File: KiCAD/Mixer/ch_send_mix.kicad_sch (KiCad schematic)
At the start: 16 parts, among them U3 NE5532, U7 NE5532

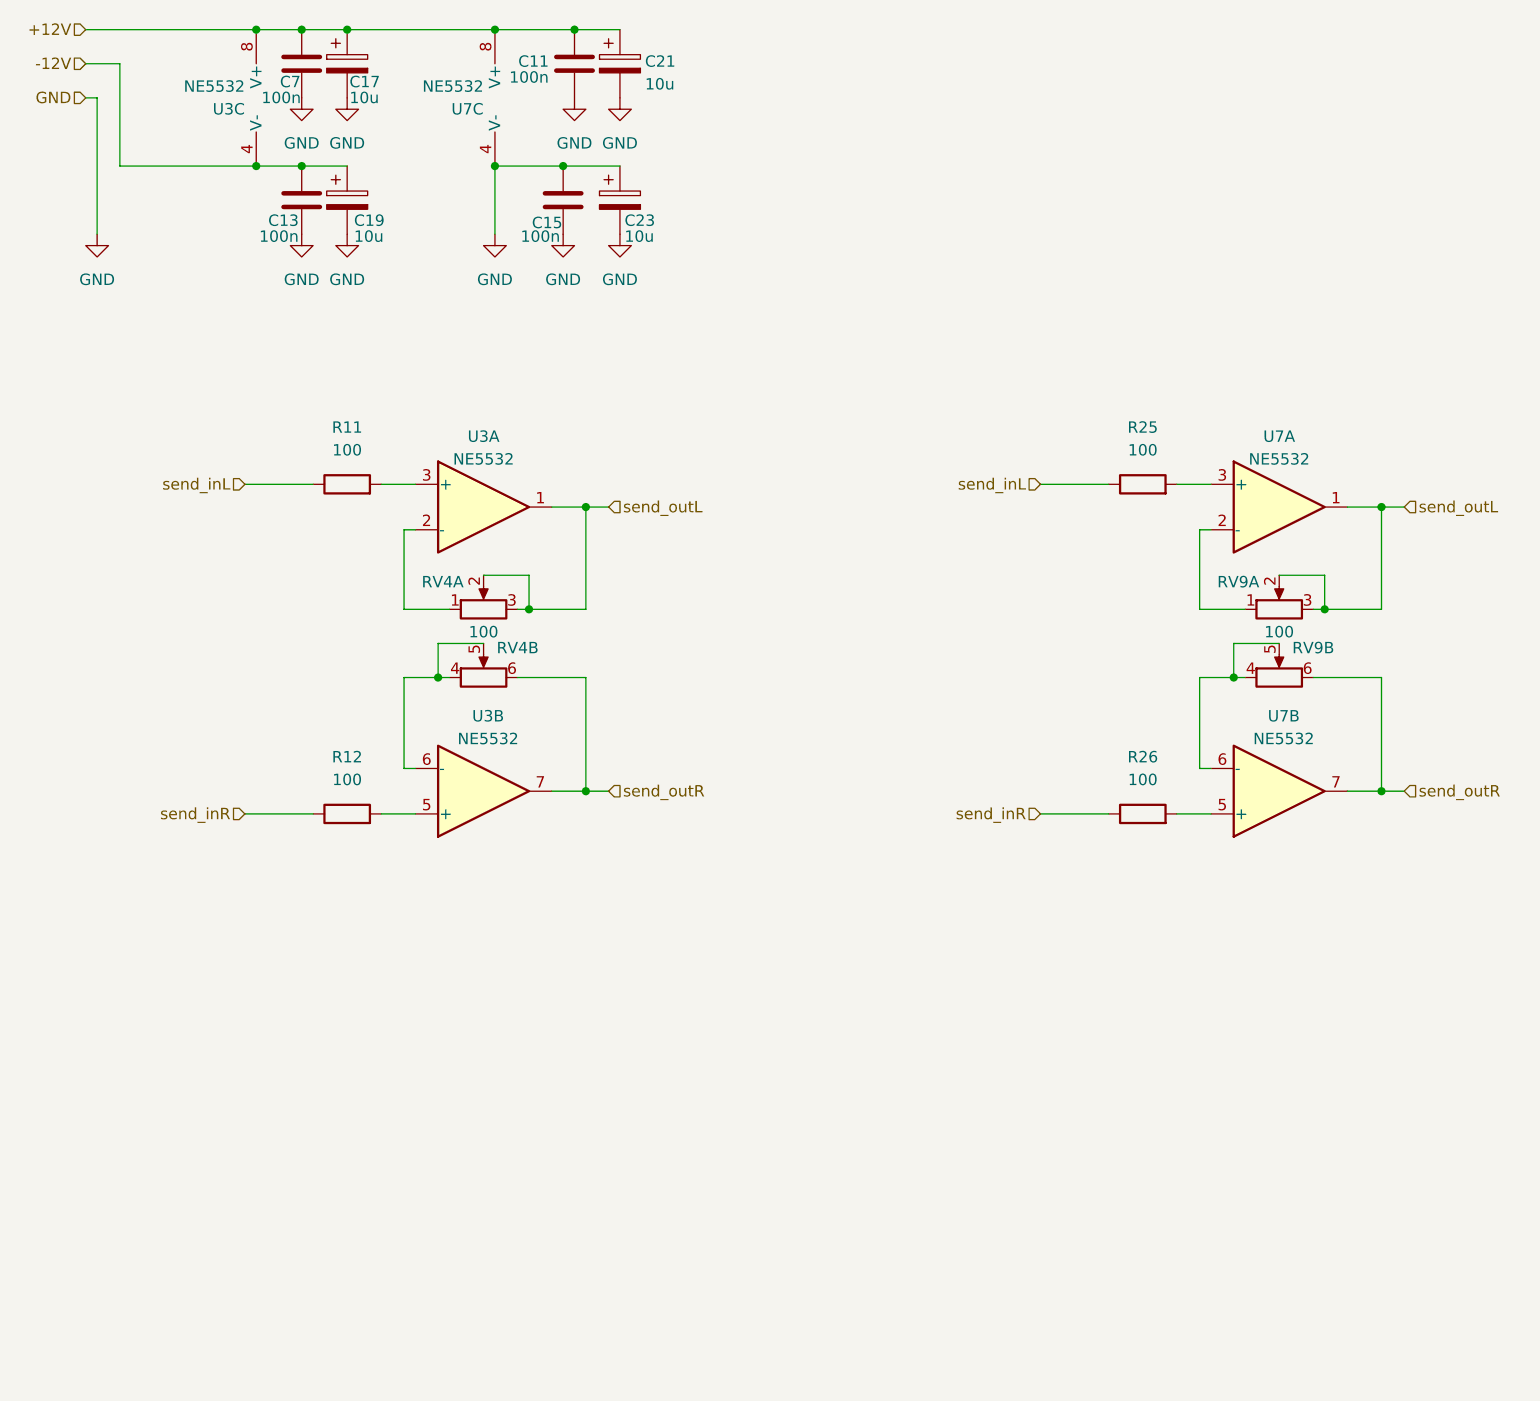
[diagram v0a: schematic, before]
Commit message: überarbeitete Schaltung und PCB Desing...v1.0 FERTIG
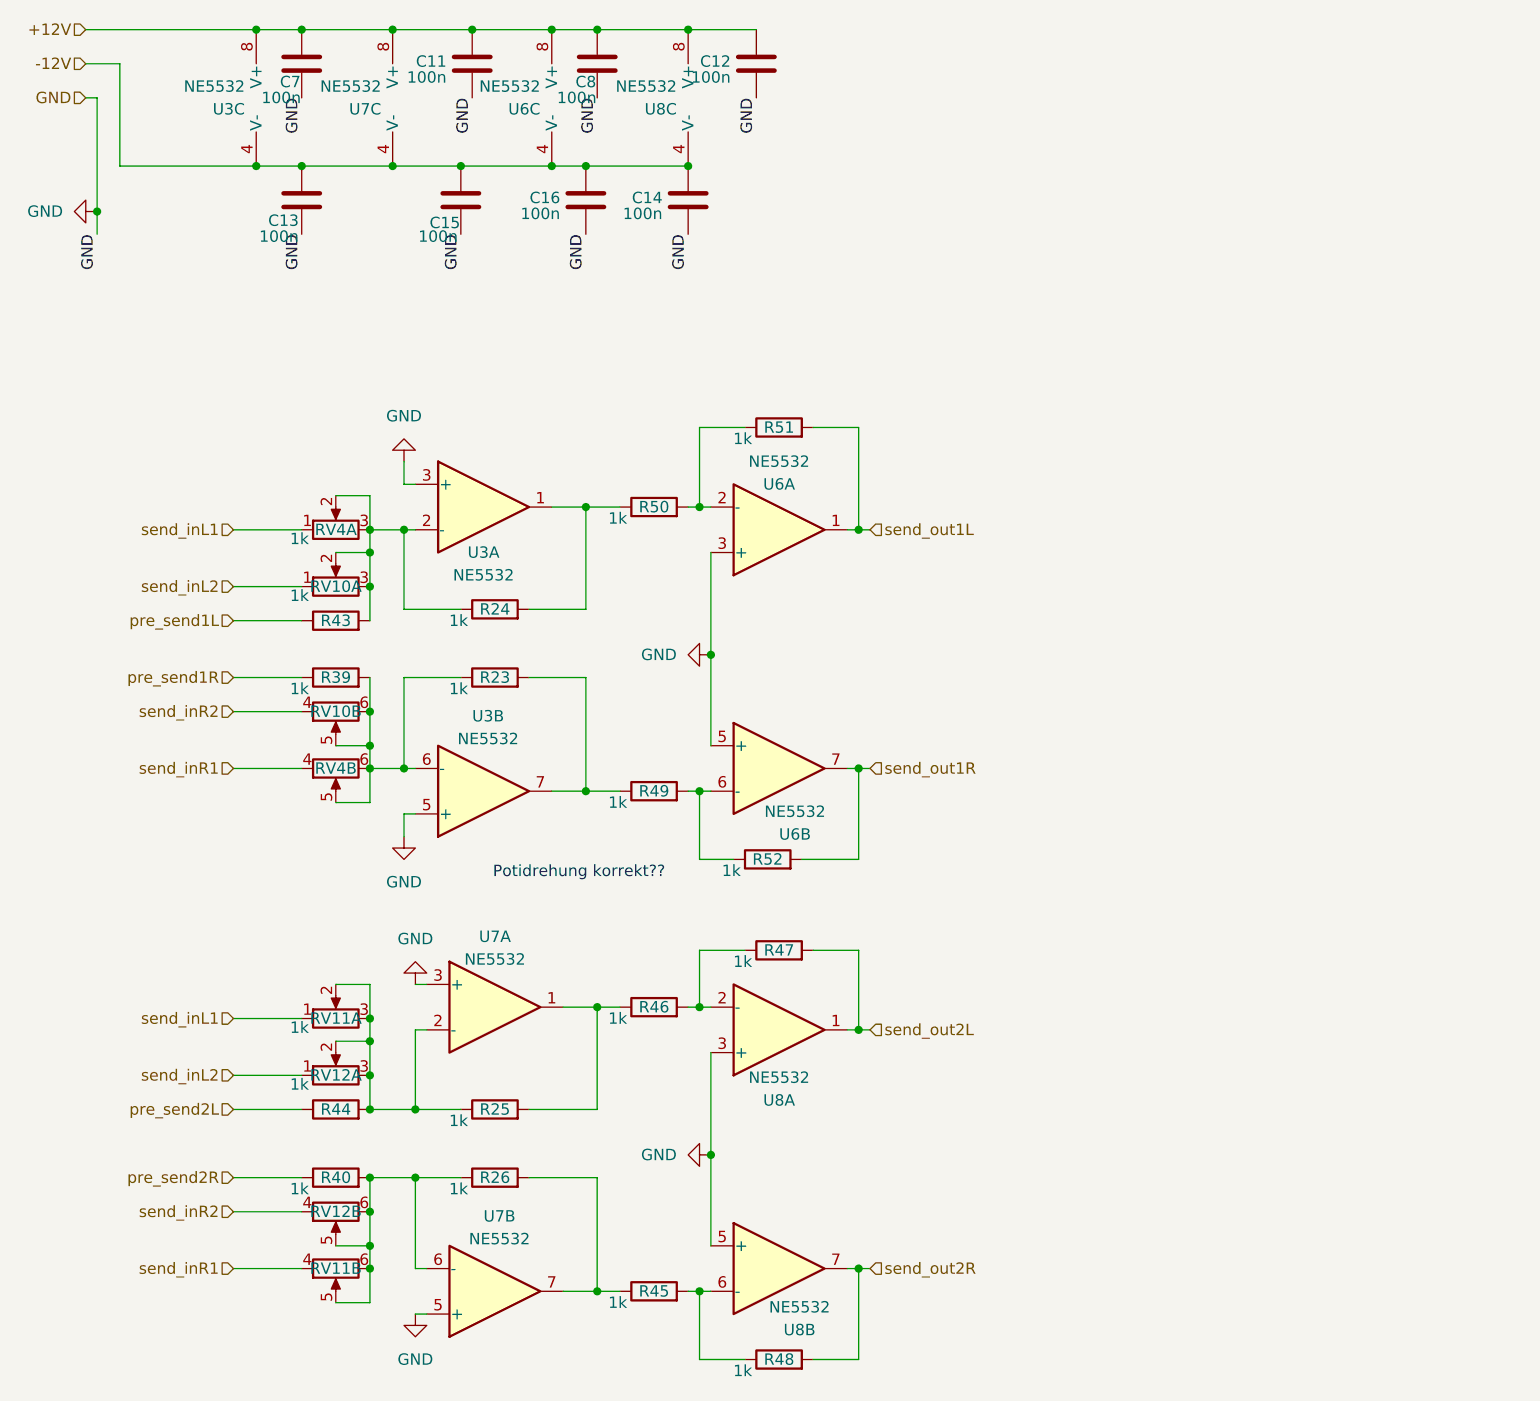
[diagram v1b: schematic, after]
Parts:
- removed C17, C19, C21, C23: 10u, Capacitor_SMD:CP_Elec_10x10, symbol Device:C_Polarized
- removed R11, R12: 100, Resistor_SMD:R_0805_2012Metric_Pad1.20x1.40mm_HandSolder, symbol Device:R
- removed RV9: 100, Potentiometer_THT:Potentiometer_Alps_RK09K_Single_Vertical, symbol Device:R_Potentiometer_Dual_Separate
- added C12, C14, C16, C8: 100n, Capacitor_SMD:C_0805_2012Metric_Pad1.18x1.45mm_HandSolder, symbol Device:C
- added R23, R24, R39, R40, R43, R44, R45, R46, R47, R48, R49, R50, R51, R52: 1k, Resistor_SMD:R_0805_2012Metric_Pad1.20x1.40mm_HandSolder, symbol Device:R
- added RV10, RV11, RV12: 1k, Potentiometer_THT:Potentiometer_Alps_RK09K_Single_Vertical, symbol Device:R_Potentiometer_Dual_Separate
- added U6, U8: NE5532, Package_SO:SOIC-8_3.9x4.9mm_P1.27mm, symbol Amplifier_Operational:NE5532
- R25, R26, RV4: value 100 -> 1k
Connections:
- net send_inL is gone; now on an unnamed net: R25.1
- net send_inR is gone; now on an unnamed net: R26.1
- net +12V: now also C12.2, C8.2, U6.8 (V+), U8.8 (V+)
- net -12V: now also C15.2, U7.4 (V-), C14.2, C16.2, U6.4 (V-), U8.4 (V-)
- net GND: now also U3.3 (+), U3.5 (+), U7.3 (+), U7.5 (+), C12.1, C14.1, C16.1, C8.1, U6.3 (+), U6.5 (+), U8.3 (+), U8.5 (+); no longer C15.2, U7.4 (V-)
- net at U7.2 (-): now also R44.2, RV11.2, RV11.3, RV12.2, RV12.3
- net at U7.6 (-): now also R40.2, RV11.5, RV11.6, RV12.5, RV12.6
- net at R25.2: now also U7.1, R46.1; no longer U7.3 (+)
- net at RV4.5, U3.6 (-): now also RV4.6, R23.1, R39.2, RV10.5, RV10.6; no longer RV4.4
- net at R26.2: now also U7.7, R45.1; no longer U7.5 (+)
- net at U3.2 (-): now also RV4.2, RV4.3, R24.1, R43.2, RV10.2, RV10.3; no longer RV4.1
- removed net send_outL: RV4.2, RV4.3, U3.1, U7.1
- removed net send_outR: RV4.6, U3.7, U7.7
- new net: R46.2, R47.1, U8.2 (-)
- new net: R23.2, R49.1, U3.7
- new net: R50.2, R51.1, U6.2 (-)
- new net: R45.2, R48.1, U8.6 (-)
- new net: R49.2, R52.1, U6.6 (-)
- new net: R24.2, R50.1, U3.1
- new net pre_send1L: R43.1
- new net pre_send1R: R39.1
- new net pre_send2L: R44.1
- new net pre_send2R: R40.1
- new net send_inL1: RV11.1, RV4.1
- new net send_inL2: RV10.1, RV12.1
- new net send_inR1: RV11.4, RV4.4
- new net send_inR2: RV10.4, RV12.4
- new net send_out1L: R51.2, U6.1
- new net send_out1R: R52.2, U6.7
- new net send_out2L: R47.2, U8.1
- new net send_out2R: R48.2, U8.7
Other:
- note added: "Potidrehung korrekt??"
- moved on the sheet: C11, C15, U7A, U7B, U7C
